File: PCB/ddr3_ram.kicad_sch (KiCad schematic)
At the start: 2 parts, among them U10 MT41J128M16JT-125K, U9 XC7A100T-CSG324

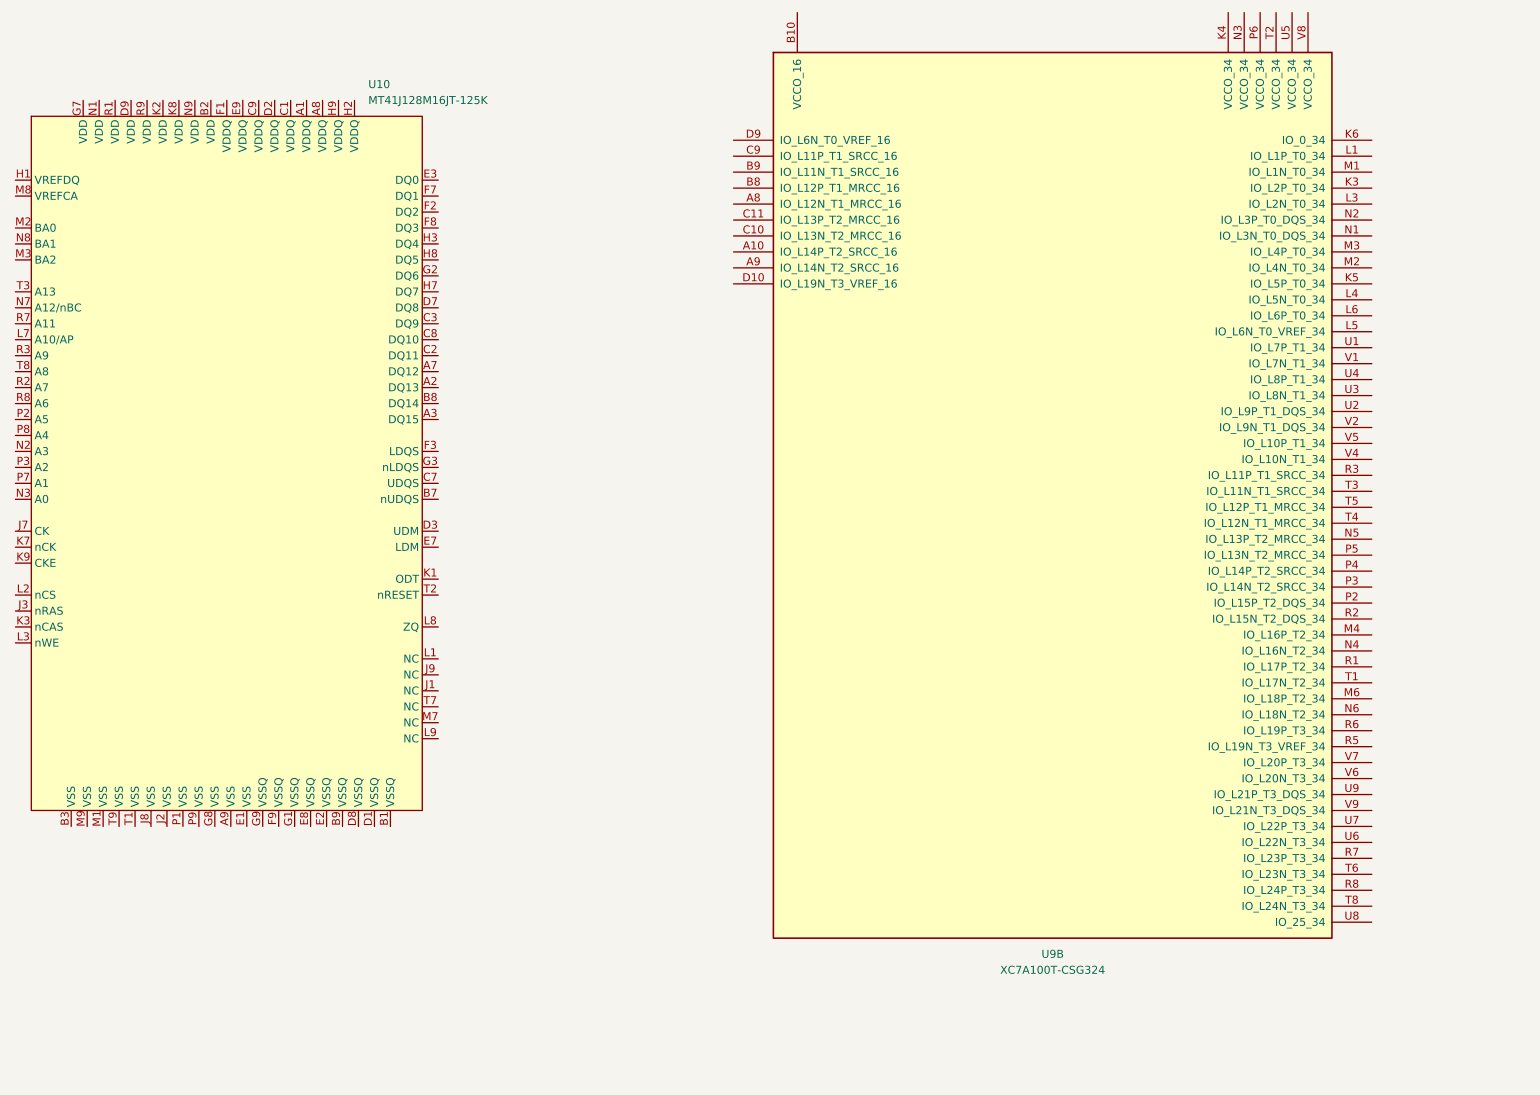
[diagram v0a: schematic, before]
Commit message: ddr wip
Signed-off-by: Kolbjørn Austreng <kolbjorn.austreng@hotzen.io>
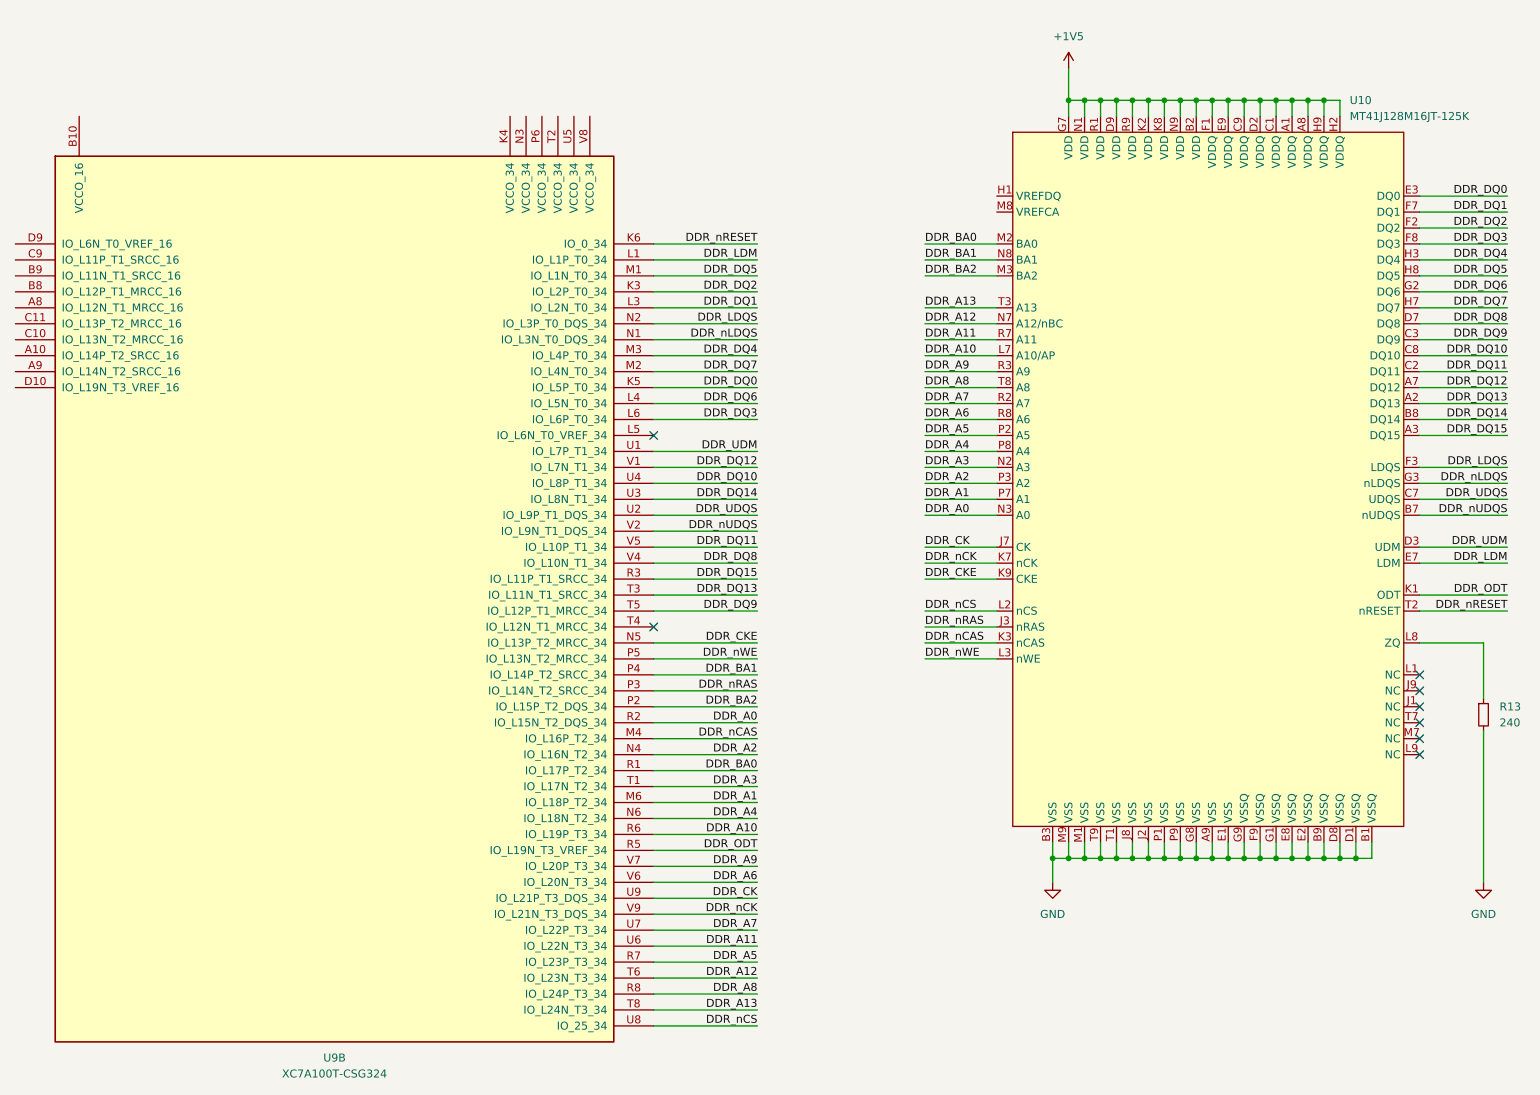
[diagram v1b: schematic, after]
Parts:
- added R13: 240, symbol Device:R_Small
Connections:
- net +1V5: now reaches U10.A1 (VDDQ)
- net +1V5: now also U10.A8 (VDDQ), U10.B2 (VDD), U10.C1 (VDDQ), U10.C9 (VDDQ), U10.D2 (VDDQ), U10.D9 (VDD), U10.E9 (VDDQ), U10.F1 (VDDQ), U10.G7 (VDD), U10.H2 (VDDQ), U10.H9 (VDDQ), U10.K2 (VDD), U10.K8 (VDD), U10.N1 (VDD), U10.N9 (VDD), U10.R1 (VDD), U10.R9 (VDD)
- net DDR_DQ13: now reaches U10.A2 (DQ13)
- net DDR_DQ13: now also U9.T3 (IO_L11N_T1_SRCC_34)
- net DDR_DQ15: now reaches U10.A3 (DQ15)
- net DDR_DQ15: now also U9.R3 (IO_L11P_T1_SRCC_34)
- net DDR_DQ12: now reaches U10.A7 (DQ12)
- net DDR_DQ12: now also U9.V1 (IO_L7N_T1_34)
- net GND: now reaches U10.A9 (VSS)
- net GND: now also U10.B1 (VSSQ), U10.B3 (VSS), U10.B9 (VSSQ), U10.D1 (VSSQ), U10.D8 (VSSQ), U10.E1 (VSS), U10.E2 (VSSQ), U10.E8 (VSSQ), U10.F9 (VSSQ), U10.G1 (VSSQ), U10.G8 (VSS), U10.G9 (VSSQ), U10.J2 (VSS), U10.J8 (VSS), U10.M1 (VSS), U10.M9 (VSS), U10.P1 (VSS), U10.P9 (VSS), U10.T1 (VSS), U10.T9 (VSS), R13.2
- net DDR_nUDQS: now reaches U10.B7 (nUDQS)
- net DDR_nUDQS: now also U9.V2 (IO_L9N_T1_DQS_34)
- net DDR_DQ14: now reaches U10.B8 (DQ14)
- net DDR_DQ14: now also U9.U3 (IO_L8N_T1_34)
- net DDR_DQ11: now reaches U10.C2 (DQ11)
- net DDR_DQ11: now also U9.V5 (IO_L10P_T1_34)
- net DDR_DQ9: now reaches U10.C3 (DQ9)
- net DDR_DQ9: now also U9.T5 (IO_L12P_T1_MRCC_34)
- net DDR_UDQS: now reaches U10.C7 (UDQS)
- net DDR_UDQS: now also U9.U2 (IO_L9P_T1_DQS_34)
- net DDR_DQ10: now reaches U10.C8 (DQ10)
- net DDR_DQ10: now also U9.U4 (IO_L8P_T1_34)
- net DDR_UDM: now reaches U10.D3 (UDM)
- net DDR_UDM: now also U9.U1 (IO_L7P_T1_34)
- net DDR_DQ8: now reaches U10.D7 (DQ8)
- net DDR_DQ8: now also U9.V4 (IO_L10N_T1_34)
- net DDR_DQ0: now reaches U10.E3 (DQ0)
- net DDR_DQ0: now also U9.K5 (IO_L5P_T0_34)
- net DDR_LDM: now reaches U10.E7 (LDM)
- net DDR_LDM: now also U9.L1 (IO_L1P_T0_34)
- net DDR_DQ2: now reaches U10.F2 (DQ2)
- net DDR_DQ2: now also U9.K3 (IO_L2P_T0_34)
- net DDR_LDQS: now reaches U10.F3 (LDQS)
- net DDR_LDQS: now also U9.N2 (IO_L3P_T0_DQS_34)
- net DDR_DQ1: now reaches U10.F7 (DQ1)
- net DDR_DQ1: now also U9.L3 (IO_L2N_T0_34)
- net DDR_DQ3: now reaches U10.F8 (DQ3)
- net DDR_DQ3: now also U9.L6 (IO_L6P_T0_34)
- net DDR_DQ6: now reaches U10.G2 (DQ6)
- net DDR_DQ6: now also U9.L4 (IO_L5N_T0_34)
- net DDR_nLDQS: now reaches U10.G3 (nLDQS)
- net DDR_nLDQS: now also U9.N1 (IO_L3N_T0_DQS_34)
- net DDR_DQ4: now reaches U10.H3 (DQ4)
- net DDR_DQ4: now also U9.M3 (IO_L4P_T0_34)
- net DDR_DQ7: now reaches U10.H7 (DQ7)
- net DDR_DQ7: now also U9.M2 (IO_L4N_T0_34)
- net DDR_DQ5: now reaches U10.H8 (DQ5)
- net DDR_DQ5: now also U9.M1 (IO_L1N_T0_34)
- net DDR_nRAS: now reaches U10.J3 (nRAS)
- net DDR_nRAS: now also U9.P3 (IO_L14N_T2_SRCC_34)
- net DDR_CK: now reaches U10.J7 (CK)
- net DDR_CK: now also U9.U9 (IO_L21P_T3_DQS_34)
- net DDR_ODT: now reaches U10.K1 (ODT)
- net DDR_ODT: now also U9.R5 (IO_L19N_T3_VREF_34)
- net DDR_nCAS: now reaches U10.K3 (nCAS)
- net DDR_nCAS: now also U9.M4 (IO_L16P_T2_34)
- net DDR_nCK: now reaches U10.K7 (nCK)
- net DDR_nCK: now also U9.V9 (IO_L21N_T3_DQS_34)
- net DDR_CKE: now reaches U10.K9 (CKE)
- net DDR_CKE: now also U9.N5 (IO_L13P_T2_MRCC_34)
- net DDR_nCS: now reaches U10.L2 (nCS)
- net DDR_nCS: now also U9.U8 (IO_25_34)
- net DDR_nWE: now reaches U10.L3 (nWE)
- net DDR_nWE: now also U9.P5 (IO_L13N_T2_MRCC_34)
- net DDR_A10: now reaches U10.L7 (A10/AP)
- net DDR_A10: now also U9.R6 (IO_L19P_T3_34)
- net at U10.L8 (ZQ): now also R13.1
- net DDR_BA0: now reaches U10.M2 (BA0)
- net DDR_BA0: now also U9.R1 (IO_L17P_T2_34)
- net DDR_BA2: now reaches U10.M3 (BA2)
- net DDR_BA2: now also U9.P2 (IO_L15P_T2_DQS_34)
- net DDR_A3: now reaches U10.N2 (A3)
- net DDR_A3: now also U9.T1 (IO_L17N_T2_34)
- net DDR_A0: now reaches U10.N3 (A0)
- net DDR_A0: now also U9.R2 (IO_L15N_T2_DQS_34)
- net DDR_A12: now reaches U10.N7 (A12/nBC)
- net DDR_A12: now also U9.T6 (IO_L23N_T3_34)
- net DDR_BA1: now reaches U10.N8 (BA1)
- net DDR_BA1: now also U9.P4 (IO_L14P_T2_SRCC_34)
- net DDR_A5: now reaches U10.P2 (A5)
- net DDR_A5: now also U9.R7 (IO_L23P_T3_34)
- net DDR_A2: now reaches U10.P3 (A2)
- net DDR_A2: now also U9.N4 (IO_L16N_T2_34)
- net DDR_A1: now reaches U10.P7 (A1)
- net DDR_A1: now also U9.M6 (IO_L18P_T2_34)
- net DDR_A4: now reaches U10.P8 (A4)
- net DDR_A4: now also U9.N6 (IO_L18N_T2_34)
- net DDR_A7: now reaches U10.R2 (A7)
- net DDR_A7: now also U9.U7 (IO_L22P_T3_34)
- net DDR_A9: now reaches U10.R3 (A9)
- net DDR_A9: now also U9.V7 (IO_L20P_T3_34)
- net DDR_A11: now reaches U10.R7 (A11)
- net DDR_A11: now also U9.U6 (IO_L22N_T3_34)
- net DDR_A6: now reaches U10.R8 (A6)
- net DDR_A6: now also U9.V6 (IO_L20N_T3_34)
- net DDR_nRESET: now reaches U10.T2 (nRESET)
- net DDR_nRESET: now also U9.K6 (IO_0_34)
- net DDR_A13: now reaches U10.T3 (A13)
- net DDR_A13: now also U9.T8 (IO_L24N_T3_34)
- net DDR_A8: now reaches U10.T8 (A8)
- net DDR_A8: now also U9.R8 (IO_L24P_T3_34)
- no-connect marks 0 -> 8
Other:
- moved on the sheet: U10, U9B
